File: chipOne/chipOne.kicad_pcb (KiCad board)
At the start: 4 copper layers, 120 x 110 mm, 27 parts

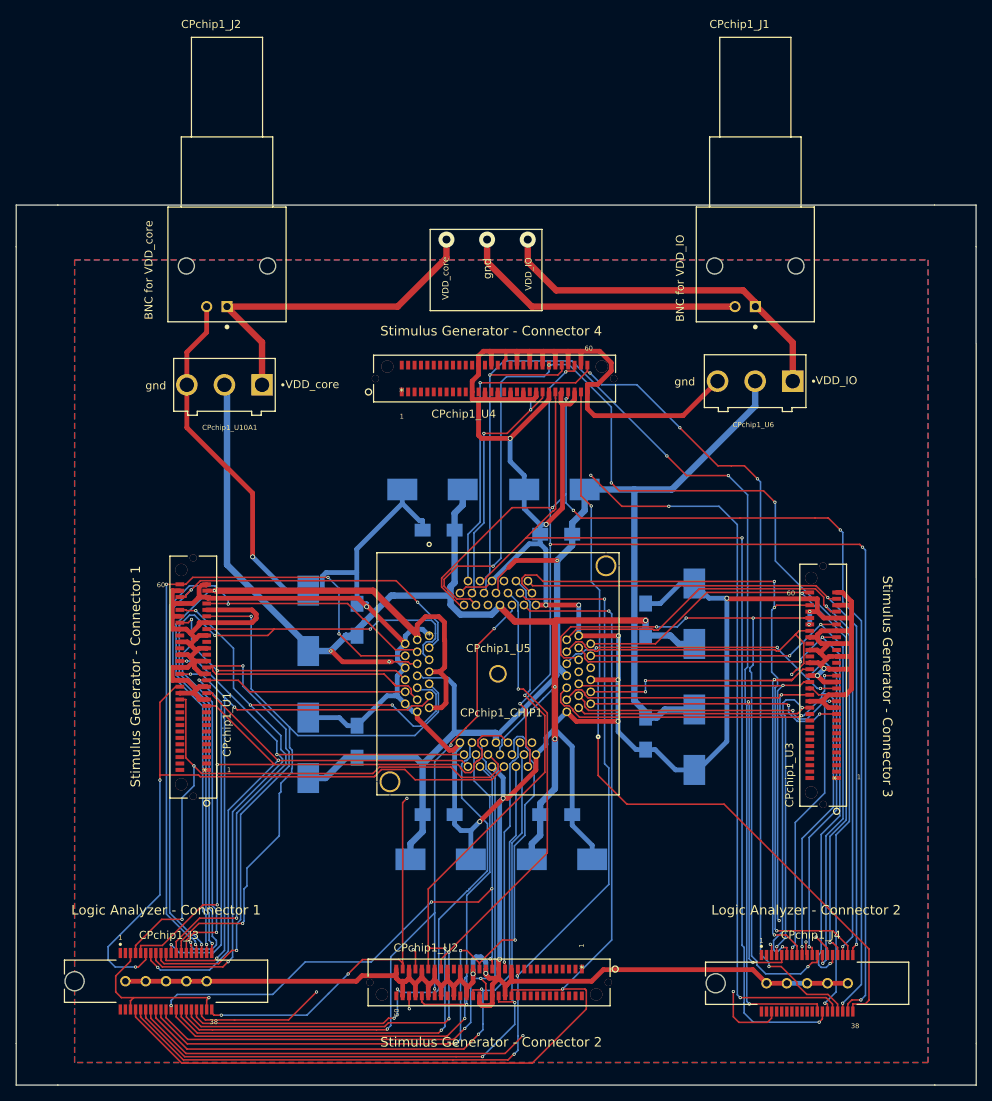
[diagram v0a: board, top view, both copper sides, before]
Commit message: Both Chips final modification done
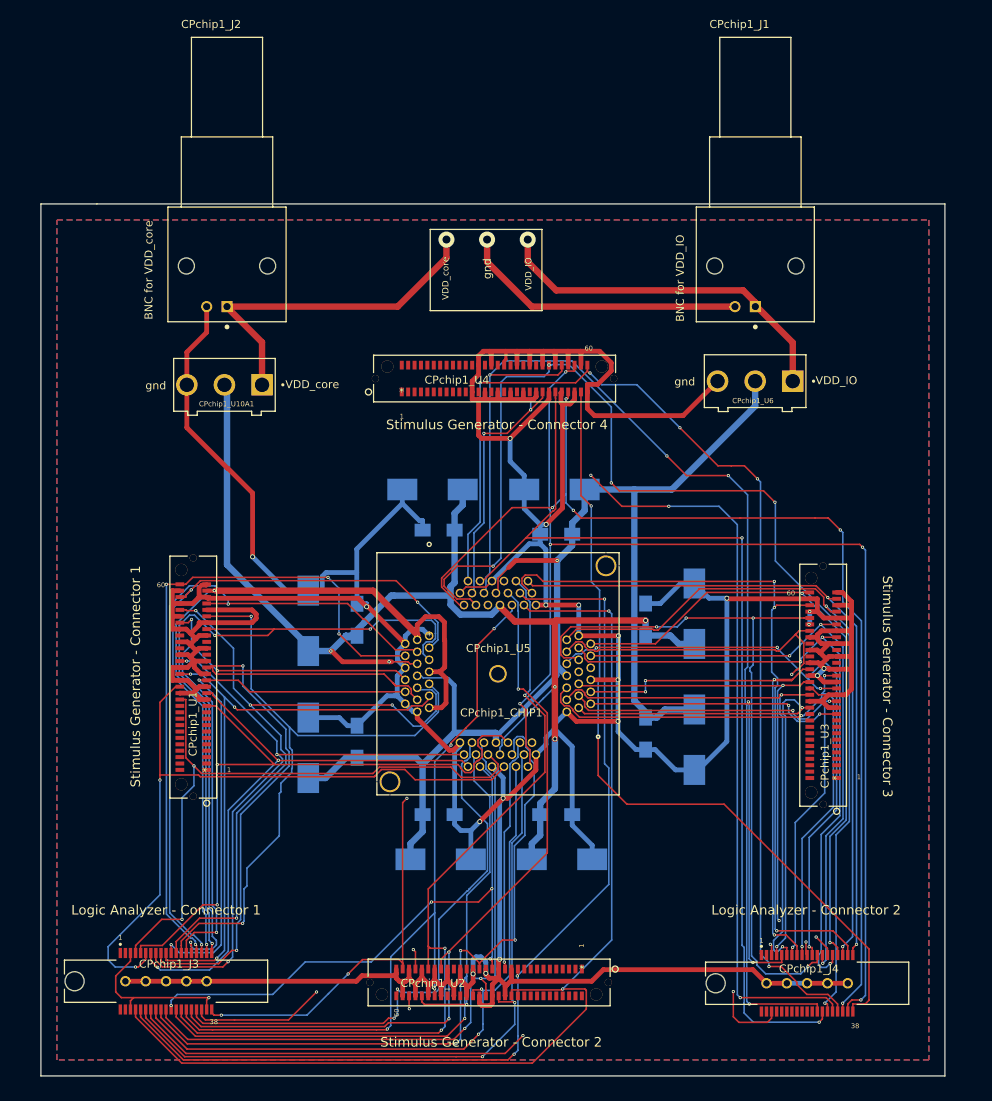
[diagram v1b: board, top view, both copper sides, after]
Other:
- board size 120 x 110 mm -> 113 x 109 mm
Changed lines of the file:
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@@
   (general
     (thickness 1.6)
-    (drawings 44)
+    (drawings 37)
     (tracks 2010)
     (zones 0)
@@
   (module Y1247AstimulusGenerator:ERF8-030-05.0-L-DV-L-TR (layer F.Cu)
     (at 45.72 110.744 270)
-    (fp_text reference CPchip1_U1 (at -5.669 -2.53 90) (layer F.SilkS)
+    (fp_text reference CPchip1_U1 (at -5.744 1.72 90) (layer F.SilkS)
       (effects (font (size 1 1) (thickness 0.15)))
     )
@@
   (module Y1247AstimulusGenerator:ERF8-030-05.0-L-DV-L-TR (layer F.Cu)
     (at 92.6211 135.636)
-    (fp_text reference CPchip1_U2 (at -19.4961 -2.661) (layer F.SilkS)
+    (fp_text reference CPchip1_U2 (at -18.6211 1.764) (layer F.SilkS)
       (effects (font (size 1 1) (thickness 0.15)))
     )
@@
   (module Y1247AstimulusGenerator:ERF8-030-05.0-L-DV-L-TR (layer F.Cu)
     (at 70.104 63.5 180)
-    (fp_text reference CPchip1_U4 (at -7.746 -2.75) (layer F.SilkS)
+    (fp_text reference CPchip1_U4 (at -6.896 1.5) (layer F.SilkS)
       (effects (font (size 1 1) (thickness 0.15)))
     )
@@
   (module Y1247AstimulusGenerator:ERF8-030-05.0-L-DV-L-TR (layer F.Cu)
     (at 124.46 111.76 270)
-    (fp_text reference CPchip1_U3 (at -0.385 5.885 90) (layer F.SilkS)
+    (fp_text reference CPchip1_U3 (at -2.76 1.46 90) (layer F.SilkS)
       (effects (font (size 1 1) (thickness 0.15)))
     )
@@
   (module U4164AlogicAnalyser:TE_5767007-8 (layer F.Cu)
     (at 40.64 137.16)
-    (fp_text reference CPchip1_J3 (at 0.36 -5.76) (layer F.SilkS)
+    (fp_text reference CPchip1_J3 (at 0.36 -2.16) (layer F.SilkS)
       (effects (font (size 1.000346 1.000346) (thickness 0.250087)))
     )
@@
   (module U4164AlogicAnalyser:TE_5767007-8 (layer F.Cu)
     (at 120.777 137.414)
-    (fp_text reference CPchip1_J4 (at 0.448 -6.039) (layer F.SilkS)
+    (fp_text reference CPchip1_J4 (at 0.223 -1.814) (layer F.SilkS)
       (effects (font (size 1.000346 1.000346) (thickness 0.250087)))
     )
@@
   (module SW_MS12ANW03:SW_MS12ANW03 (layer F.Cu)
     (at 114.28 62.15 180)
-    (fp_text reference CPchip1_U6 (at 0.23 -5.45) (layer F.SilkS)
+    (fp_text reference CPchip1_U6 (at 0.28 -2.45) (layer F.SilkS)
       (effects (font (size 0.64 0.64) (thickness 0.16)))
     )
@@
   (module SW_MS12ANW03:SW_MS12ANW03 (layer F.Cu)
     (at 47.94 62.61 180)
-    (fp_text reference CPchip1_U10A1 (at -0.66 -5.34) (layer F.SilkS)
+    (fp_text reference CPchip1_U10A1 (at -0.26 -2.39) (layer F.SilkS)
       (effects (font (size 0.64 0.64) (thickness 0.16)))
     )
@@
       (net 2 VSSQ))
   )
+  (gr_line (start 25 40) (end 25 149) (layer Edge.Cuts) (width 0.05))
+  (gr_line (start 32 40) (end 25 40) (layer Edge.Cuts) (width 0.05))
+  (gr_line (start 138 40) (end 32 40) (layer Edge.Cuts) (width 0.05))
+  (gr_line (start 138 149) (end 138 40) (layer Edge.Cuts) (width 0.05))
+  (gr_line (start 25 149) (end 138 149) (layer Edge.Cuts) (width 0.05))
   (gr_text gnd (at 105.48 62.22) (layer F.SilkS)
     (effects (font (size 1 1) (thickness 0.2)))
@@
     (effects (font (size 1 1) (thickness 0.25)))
   )
-  (gr_line (start 21.91 150.14) (end 27.11 150.14) (layer Edge.Cuts) (width 0.05))
-  (gr_line (start 21.91 144.94) (end 21.91 150.14) (layer Edge.Cuts) (width 0.05))
-  (gr_line (start 21.91 40.14) (end 27.11 40.14) (layer Edge.Cuts) (width 0.05))
-  (gr_line (start 21.91 45.34) (end 21.91 40.14) (layer Edge.Cuts) (width 0.05))
-  (gr_line (start 141.9 40.14) (end 141.9 45.34) (layer Edge.Cuts) (width 0.05))
-  (gr_line (start 136.7 40.14) (end 141.9 40.14) (layer Edge.Cuts) (width 0.05))
-  (gr_line (start 141.92 150.14) (end 141.92 144.94) (layer Edge.Cuts) (width 0.05))
-  (gr_line (start 136.72 150.14) (end 141.92 150.14) (layer Edge.Cuts) (width 0.05))
-  (gr_text "PCB Designed for Chip 1" (at 123.825 145.415) (layer B.SilkS)
+  (gr_text "PCB Designed for Chip 1" (at 123 147) (layer B.SilkS)
     (effects (font (size 1.5 1.5) (thickness 0.3)) (justify mirror))
   )
@@
     (effects (font (size 1.2 1.2) (thickness 0.25)))
   )
-  (gr_text "Stimulus Generator - Connector 4" (at 81.28 55.88) (layer F.SilkS)
+  (gr_text "Stimulus Generator - Connector 4" (at 82 67.6) (layer F.SilkS)
     (effects (font (size 1.2 1.2) (thickness 0.25)))
   )
@@
     (effects (font (size 1.2 1.2) (thickness 0.25)))
   )
-  (gr_line (start 21.91 45.34) (end 21.91 144.94) (layer Edge.Cuts) (width 0.05))
-  (gr_line (start 27.11 40.14) (end 136.7 40.14) (layer Edge.Cuts) (width 0.05))
-  (gr_line (start 141.92 144.94) (end 141.9 45.34) (layer Edge.Cuts) (width 0.05))
-  (gr_line (start 136.72 150.14) (end 27.11 150.14) (layer Edge.Cuts) (width 0.05))
   (segment (start 81.8809 107.3279) (end 81.8809 106.171) (width 0.8) (layer B.Cu) (net 1))
   (segment (start 81.8809 107.328) (end 81.8809 107.3279) (width 0.8) (layer B.Cu) (net 1))
@@
   (segment (start 92.2274 98.740398) (end 92.2274 98.480001) (width 0.2) (layer In1.Cu) (net 3))
   (segment (start 91.233899 99.733899) (end 92.2274 98.740398) (width 0.2) (layer In1.Cu) (net 3))
-  (via (at 85.852 44.45) (size 2) (drill 1) (layers F.Cu B.Cu) (net 60))
-  (segment (start 114.3 52.832) (end 114.3 52.324) (width 0.8) (layer F.Cu) (net 60))
-  (segment (start 114.3 52.324) (end 112.776 50.8) (width 0.8) (layer F.Cu) (net 60))
-  (segment (start 112.776 50.8) (end 89.408 50.8) (width 0.8) (layer F.Cu) (net 60))
-  (segment (start 85.852 47.244) (end 85.852 44.45) (width 0.8) (layer F.Cu) (net 60))
-  (segment (start 89.408 50.8) (end 85.852 47.244) (width 0.8) (layer F.Cu) (net 60))
-  (segment (start 114.3 52.832) (end 114.482 52.832) (width 0.8) (layer F.Cu) (net 60))
-  (segment (start 118.98 57.33) (end 118.98 62.15) (width 0.8) (layer F.Cu) (net 60))
-  (segment (start 114.482 52.832) (end 118.98 57.33) (width 0.8) (layer F.Cu) (net 60))
-  (via (at 75.692 44.45) (size 2) (drill 1) (layers F.Cu B.Cu) (net 61))
-  (segment (start 75.692 46.736) (end 75.692 44.45) (width 0.8) (layer F.Cu) (net 61))
-  (segment (start 48.26 52.832) (end 69.596 52.832) (width 0.8) (layer F.Cu) (net 61))
-  (segment (start 69.596 52.832) (end 75.692 46.736) (width 0.8) (layer F.Cu) (net 61))
-  (segment (start 48.26 52.832) (end 48.26 52.91) (width 0.8) (layer F.Cu) (net 61))
-  (segment (start 52.64 57.29) (end 52.64 62.61) (width 0.8) (layer F.Cu) (net 61))
-  (segment (start 48.26 52.91) (end 52.64 57.29) (width 0.8) (layer F.Cu) (net 61))
   (segment (start 54.1833 110.07) (end 47.042 110.07) (width 0.2) (layer F.Cu) (net 4))
   (segment (start 47.042 127.6091) (end 47.042 110.07) (width 0.2) (layer B.Cu) (net 4))
@@
   (segment (start 86.2245 66.4008) (end 93.7411 73.9174) (width 0.2) (layer In1.Cu) (net 59))
   (segment (start 86.2245 65.7281) (end 86.2245 66.4008) (width 0.2) (layer In1.Cu) (net 59))
+  (via (at 85.852 44.45) (size 2) (drill 1) (layers F.Cu B.Cu) (net 60))
+  (segment (start 114.3 52.832) (end 114.3 52.324) (width 0.8) (layer F.Cu) (net 60))
+  (segment (start 114.3 52.324) (end 112.776 50.8) (width 0.8) (layer F.Cu) (net 60))
+  (segment (start 112.776 50.8) (end 89.408 50.8) (width 0.8) (layer F.Cu) (net 60))
+  (segment (start 85.852 47.244) (end 85.852 44.45) (width 0.8) (layer F.Cu) (net 60))
+  (segment (start 89.408 50.8) (end 85.852 47.244) (width 0.8) (layer F.Cu) (net 60))
+  (segment (start 114.3 52.832) (end 114.482 52.832) (width 0.8) (layer F.Cu) (net 60))
+  (segment (start 118.98 57.33) (end 118.98 62.15) (width 0.8) (layer F.Cu) (net 60))
+  (segment (start 114.482 52.832) (end 118.98 57.33) (width 0.8) (layer F.Cu) (net 60))
+  (via (at 75.692 44.45) (size 2) (drill 1) (layers F.Cu B.Cu) (net 61))
+  (segment (start 75.692 46.736) (end 75.692 44.45) (width 0.8) (layer F.Cu) (net 61))
+  (segment (start 48.26 52.832) (end 69.596 52.832) (width 0.8) (layer F.Cu) (net 61))
+  (segment (start 69.596 52.832) (end 75.692 46.736) (width 0.8) (layer F.Cu) (net 61))
+  (segment (start 48.26 52.832) (end 48.26 52.91) (width 0.8) (layer F.Cu) (net 61))
+  (segment (start 52.64 57.29) (end 52.64 62.61) (width 0.8) (layer F.Cu) (net 61))
+  (segment (start 48.26 52.91) (end 52.64 57.29) (width 0.8) (layer F.Cu) (net 61))
   (zone (net 2) (net_name VSSQ) (layer F.Cu) (hatch edge 0.508)
     (connect_pads (clearance 0.8))
@@
     (polygon
       (pts
-        (xy 135.89 147.32) (xy 29.21 147.32) (xy 29.21 46.99) (xy 135.89 46.99)
+        (xy 136 147) (xy 27 147) (xy 27 42) (xy 136 42)
       )
     )
@@
     (polygon
       (pts
-        (xy 135.89 147.32) (xy 29.21 147.32) (xy 29.21 46.99) (xy 135.89 46.99)
+        (xy 136 147) (xy 27 147) (xy 27 42) (xy 136 42)
       )
     )
